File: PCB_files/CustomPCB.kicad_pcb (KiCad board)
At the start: 2 copper layers, 72.4 x 54.6 mm, 11 parts, among them M2.5 MountingHole_2.7mm_M2.5

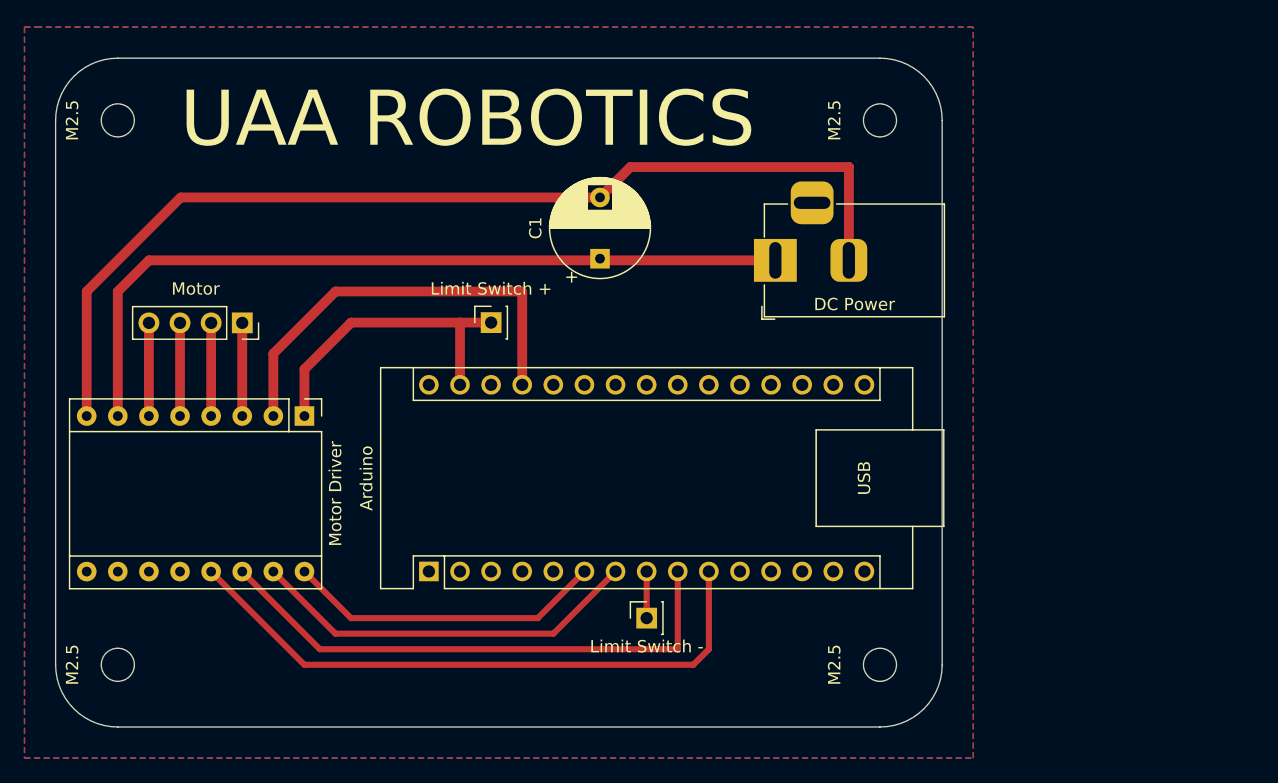
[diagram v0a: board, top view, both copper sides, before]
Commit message: PCB V2
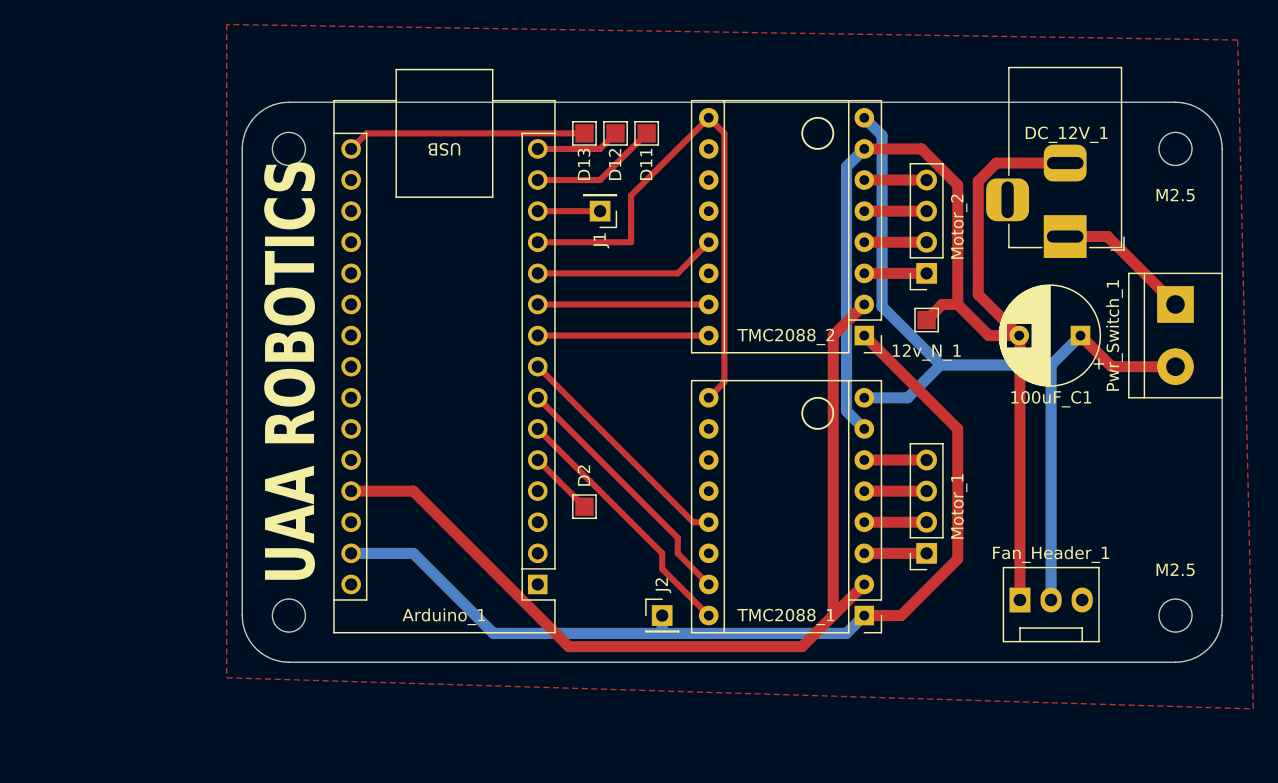
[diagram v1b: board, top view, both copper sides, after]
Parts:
- removed Arduino: Arduino_Nano_v3.x, Module:Arduino_Nano
- removed C1: C 100, Capacitor_THT:CP_Radial_D8.0mm_P5.00mm
- removed DC Power: Barrel_Jack_MountingPin, Connector_BarrelJack:BarrelJack_Horizontal
- removed Limit Switch +: Conn_01x01_Socket, Connector_PinSocket_2.54mm:PinSocket_1x01_P2.54mm_Vertical
- removed Limit Switch -: Conn_01x01_Socket, Connector_PinSocket_2.54mm:PinSocket_1x01_P2.54mm_Vertical
- removed the M2.5 at (174.0, 73.9)
- removed the M2.5 at (111.8, 118.3)
- removed the M2.5 at (174.0, 118.3)
- removed the M2.5 at (111.8, 73.9)
- removed Motor: Conn_01x04_Socket, Connector_PinSocket_2.54mm:PinSocket_1x04_P2.54mm_Vertical
- removed Motor Driver: Pololu_Breakout_A4988, Module:Pololu_Breakout-16_15.2x20.3mm
- added 100uF_C1: C 100, Capacitor_THT:CP_Radial_D8.0mm_P5.00mm, F.Cu at (190.4, 91.4)
- added 12v_N_1: TestPoint, TestPoint:TestPoint_Pad_1.5x1.5mm, F.Cu at (177.8, 90.2)
- added Arduino_1: Arduino_Nano_v3.x, Module:Arduino_Nano, F.Cu at (146.1, 111.8)
- added D11: TestPoint, TestPoint:TestPoint_Pad_1.5x1.5mm, F.Cu at (154.9, 74.9)
- added D12: TestPoint, TestPoint:TestPoint_Pad_1.5x1.5mm, F.Cu at (152.4, 74.9)
- added D13: TestPoint, TestPoint:TestPoint_Pad_1.5x1.5mm, F.Cu at (149.9, 74.9)
- added D2: TestPoint, TestPoint:TestPoint_Pad_1.5x1.5mm, F.Cu at (149.9, 105.4)
- added DC_12V_1: Barrel_Jack_MountingPin, Connector_BarrelJack:BarrelJack_Horizontal, F.Cu at (189.1, 83.4)
- added Fan_Header_1: Fan_3pin, Connector:FanPinHeader_1x03_P2.54mm_Vertical, F.Cu at (185.4, 113.0)
- added J1: Limit 1x1 Pin, Connector_PinHeader_2.54mm:PinHeader_1x01_P2.54mm_Vertical, F.Cu at (151.1, 81.3)
- added J2: Conn_01x01_Socket, Connector_PinHeader_2.54mm:PinHeader_1x01_P2.54mm_Vertical, F.Cu at (156.2, 114.3)
- added M2.5: MountingHole_2.7mm_M2.5, MountingHole:MountingHole_2.7mm_M2.5, F.Cu at (198.1, 76.2)
- added M2.5: MountingHole_2.7mm_M2.5, MountingHole:MountingHole_2.7mm_M2.5, F.Cu at (198.1, 114.3)
- added M2.5: MountingHole_2.7mm_M2.5, MountingHole:MountingHole_2.7mm_M2.5, F.Cu at (125.7, 114.3)
- added M2.5: MountingHole_2.7mm_M2.5, MountingHole:MountingHole_2.7mm_M2.5, F.Cu at (125.7, 76.2)
- added Motor_1: Conn_01x04_Socket, Connector_PinSocket_2.54mm:PinSocket_1x04_P2.54mm_Vertical, F.Cu at (177.8, 109.2)
- added Motor_2: Conn_01x04_Socket, Connector_PinSocket_2.54mm:PinSocket_1x04_P2.54mm_Vertical, F.Cu at (177.8, 86.4)
- added Pwr_Switch_1: Screw_Terminal_01x02, TerminalBlock:TerminalBlock_bornier-2_P5.08mm, F.Cu at (198.1, 88.9)
- added TMC2088_1: Pololu_Breakout_A4988, Module:Pololu_Breakout-16_15.2x20.3mm, F.Cu at (172.7, 114.3)
- added TMC2088_2: Pololu_Breakout_A4988, Module:Pololu_Breakout-16_15.2x20.3mm, F.Cu at (172.7, 91.4)
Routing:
- net /12v Negative: track 0.00 -> 95.1 mm
- net /5v Positive: track 84.2 -> 0.00 mm
- net /12v Positive: track 0.00 -> 70.7 mm
- net /5v Negative: track 64.9 -> 0.00 mm
- net /Logic Negative: track 25.7 -> 77.6 mm
- net /Signal1: track 50.7 -> 0.00 mm
- net /Signal2: track 44.5 -> 0.00 mm
- net /Enable Pin: track 0.00 -> 44.3 mm
- net /Logic Positive: track 35.1 -> 75.7 mm
- net /Signal3: track 32.1 -> 0.00 mm
- net /Signal4: track 26.0 -> 0.00 mm
- net /Step2: track 0.00 -> 21.0 mm
- net /Direction2: track 0.00 -> 21.0 mm
- net /D13 Breakout: track 0.00 -> 19.6 mm
- net /Reset2: track 0.00 -> 19.2 mm
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- removed copper zone on B.Cu, net (none)
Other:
- board size 72.4 x 54.6 mm -> 80 x 45.7 mm
